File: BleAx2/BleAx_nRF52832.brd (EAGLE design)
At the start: 30 x 20.1 mm, 42 parts, among them CN1 6p-2.54, J1 2.0MM-90D, U1 NRF52832, U2 MCP73832T-2ACI/OT-SOT23-5, U4 MIC5225-3.3, X1 FA-128, X2 32.768kHz

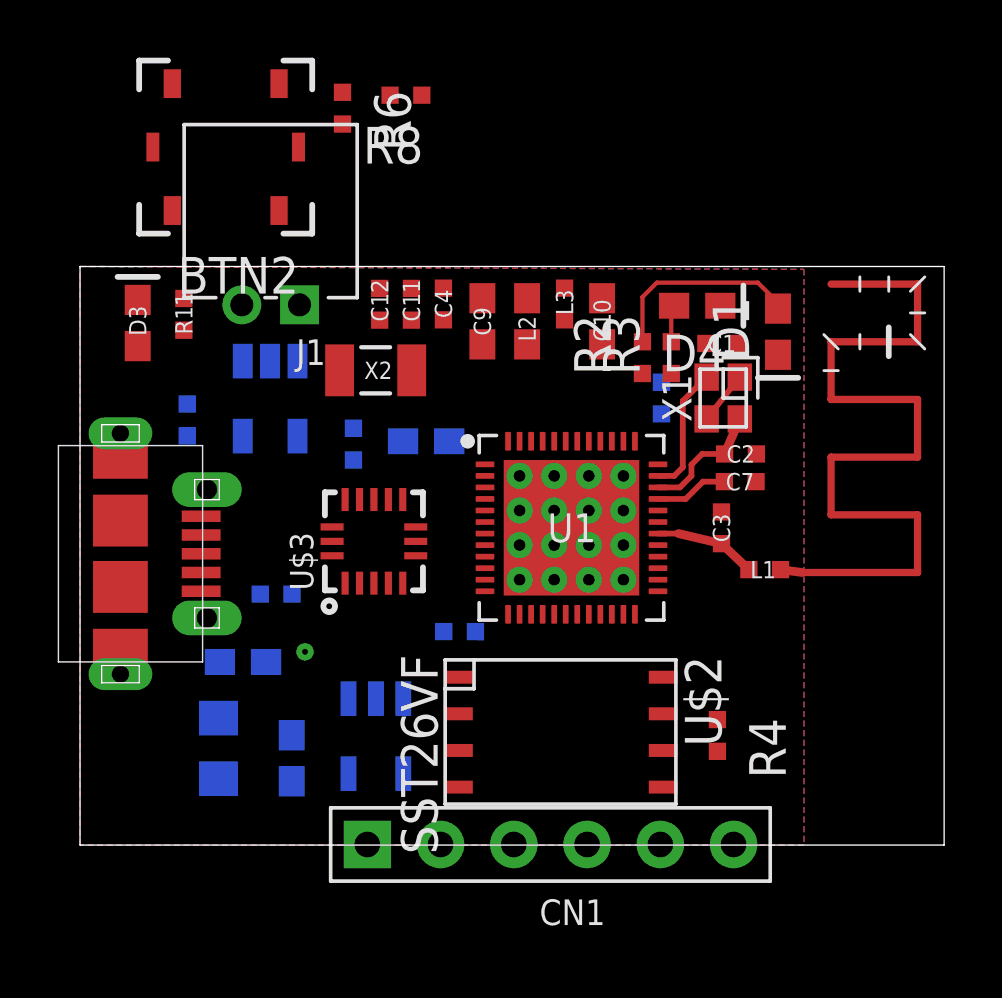
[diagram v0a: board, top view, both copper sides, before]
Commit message: halfway?
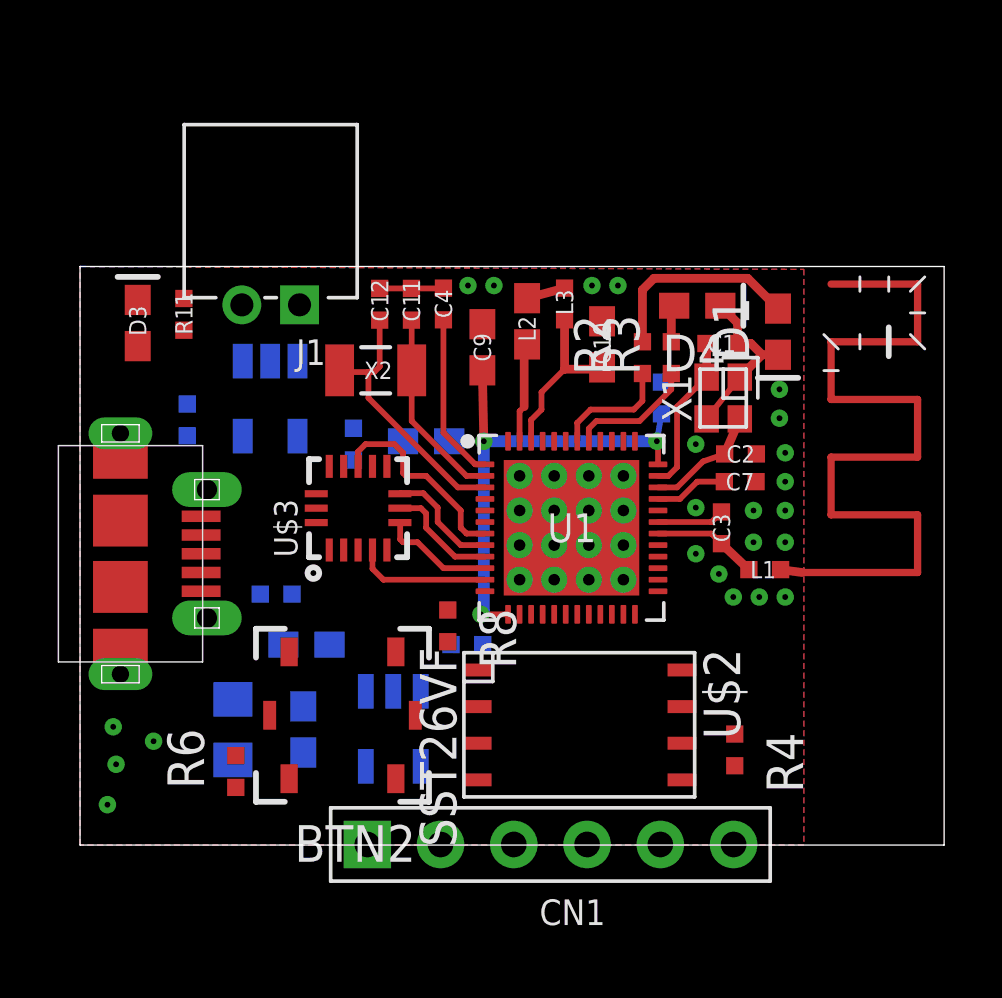
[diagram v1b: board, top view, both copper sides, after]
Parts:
- moved R6 23.3 mm to (5.40, 2.55), turned to 90 degrees
- moved BTN2 20.1 mm to (9.10, 4.50)
- moved R8 18.5 mm to (12.8, 7.60), turned to 270 degrees
- moved C17 2.28 mm to (7.85, 6.95)
- moved U$3 1.27 mm to (9.64, 11.7)
- moved C6 1.08 mm to (7.74, 4.01)
- moved C9 0.90 mm to (13.9, 17.3)
- moved C19 0.82 mm to (5.30, 4.05)
- moved C10 0.80 mm to (18.1, 17.4)
- moved R4 0.78 mm to (22.7, 3.30)
- moved U$2 0.70 mm to (17.5, 4.10)
- moved U4 0.65 mm to (10.9, 4.03)
- moved C5 0.51 mm to (13.4, 6.95)
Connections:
- net BTTN_01: now also U1.12; no longer U1.43
- net LIS_CS: now also U1.8; no longer U1.9
- net LIS_INT1: now also U1.7; no longer U1.8
- net MISO_01: now also U1.9; no longer U1.10
- net MOSI_01: now also U1.10; no longer U1.11
- net SCK_01: now also U1.11; no longer U1.12
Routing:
- net VDD_P3V3: track 0.23 -> 17.2 mm, vias 0 -> 3
- net XL2: track 0.00 -> 9.33 mm
- net GND: track 1.85 -> 10.6 mm, vias 0 -> 23
- net LIS_INT1: track 0.00 -> 7.06 mm
- net XL1: track 0.00 -> 6.83 mm
- net DEC4: track 0.00 -> 6.02 mm
- net DEC1: track 0.00 -> 5.81 mm
- net SCK_01: track 0.00 -> 4.71 mm
- net LED_02: track 0.00 -> 4.41 mm
- net LED_01: track 0.00 -> 4.16 mm
- net LIS_CS: track 0.00 -> 4.00 mm
- net MISO_01: track 0.00 -> 3.94 mm
- net MOSI_01: track 0.00 -> 3.94 mm
- net N$4: track 0.00 -> 3.47 mm
- net N$2: track 0.00 -> 1.35 mm
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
